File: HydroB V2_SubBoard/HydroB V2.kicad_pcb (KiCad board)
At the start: 4 copper layers, 89.6 x 101.8 mm, 77 parts, among them J1 FAN, J14 Screw_Terminal_01x02, J15 Screw_Terminal_01x02, J16 Screw_Terminal_01x02, J17 Screw_Terminal_01x02, J18 Screw_Terminal_01x02, J3 Conn_01x02_Pin, J4 Conn_01x04_Pin, J5 PH SENSOR, J6 EC SENSOR, J7 Conn_01x02_Pin, K10 SRD-05VDC-SL-C, K5 SRD-05VDC-SL-C, K7 SRD-05VDC-SL-C, K8 SRD-05VDC-SL-C, K9 SRD-05VDC-SL-C, Q10 S8050, Q6 S8050, Q7 S8050, Q8 S8050, Q9 S8050, SW1 SW_Push, U1 STM32F103C8Tx, U2 TPS5410D, U3 SN65HVD72DR, U4 TPS7A2633DRVR, U5 SN65HVD230, Y1 8Mhz

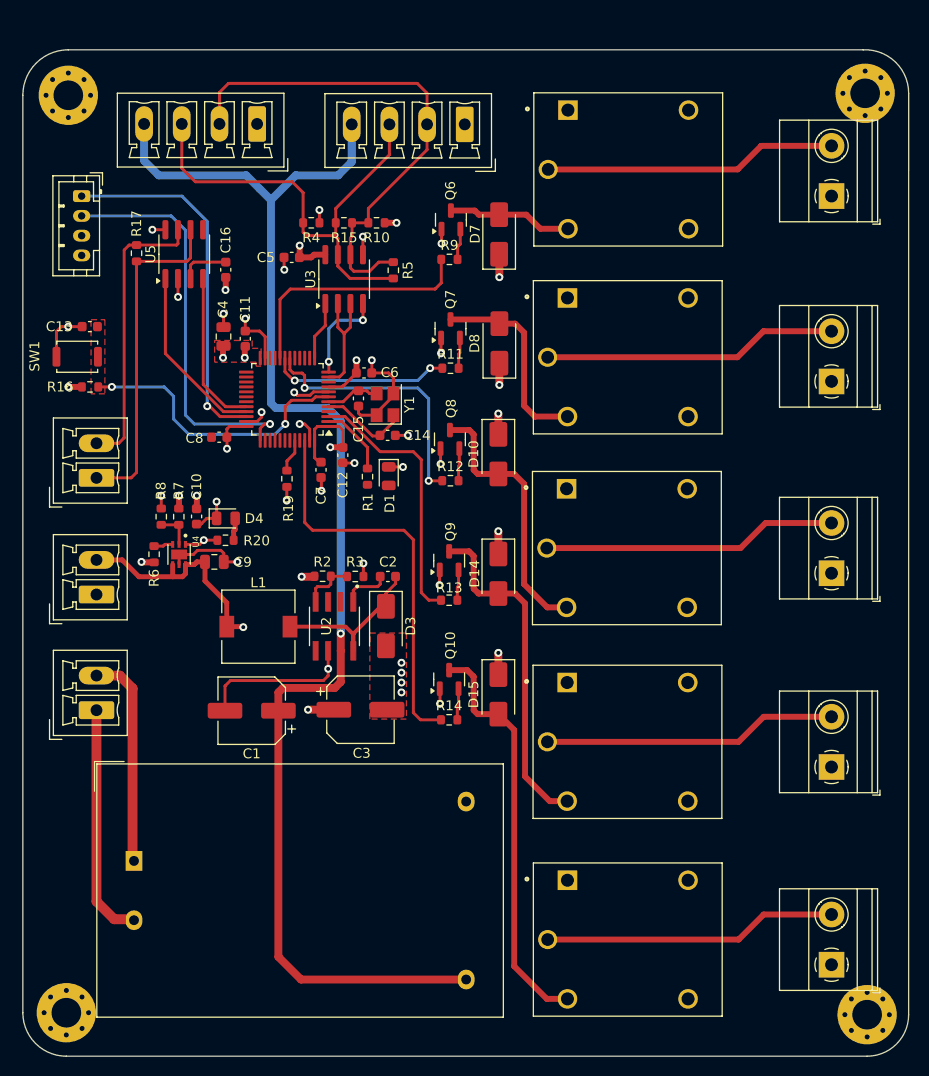
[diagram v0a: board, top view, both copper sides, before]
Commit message: finish the subboard layout
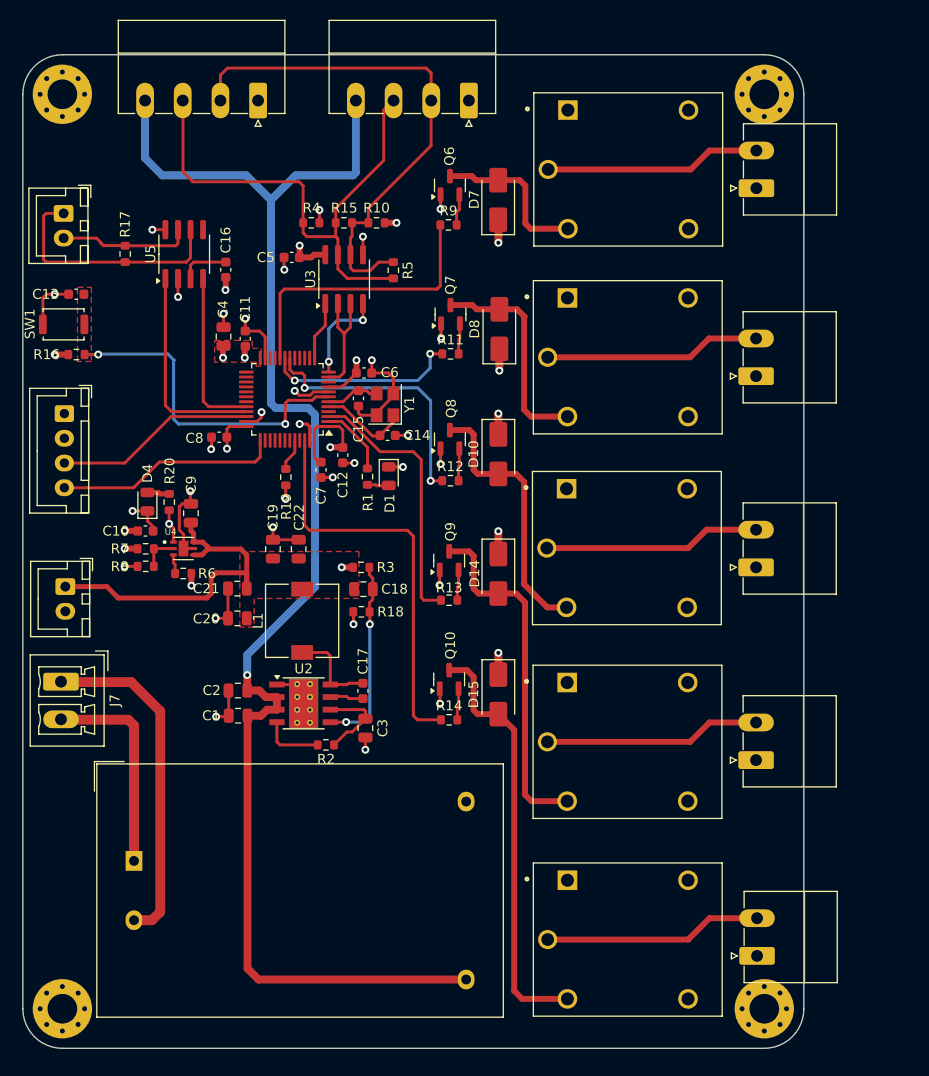
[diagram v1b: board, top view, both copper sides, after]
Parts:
- removed D3: B340, Diode_SMD:D_SMA
- removed J3: Conn_01x02_Pin, Connector_Phoenix_MC:PhoenixContact_MCV_1,5_2-G-3.5_1x02_P3.50mm_Vertical
- added C17: 0.1uF, Capacitor_SMD:C_0603_1608Metric, F.Cu at (138.4, 109.8)
- added C18: c, Capacitor_SMD:C_0805_2012Metric, F.Cu at (138.4, 99.6)
- added C19: 22uF, Capacitor_SMD:C_0805_2012Metric, F.Cu at (129.3, 95.5)
- added C20: 22uF, Capacitor_SMD:C_0805_2012Metric, F.Cu at (125.7, 102.5)
- added C21: 22uF, Capacitor_SMD:C_0805_2012Metric, F.Cu at (125.7, 99.5)
- added C22: 22uF, Capacitor_SMD:C_0805_2012Metric, F.Cu at (131.9, 95.5)
- added J2: Conn_01x02_Pin, Connector_JST:JST_XH_B2B-XH-A_1x02_P2.50mm_Vertical, F.Cu at (108.3, 99.3)
- added R18: 9.09k, Resistor_SMD:R_0603_1608Metric, F.Cu at (138.2, 101.8)
- C1: value 4.7uF -> 10uF; footprint Capacitor_SMD:CP_Elec_6.3x5.4_Nichicon -> Capacitor_SMD:C_0805_2012Metric
- C2: value 0.01uF -> 220nF; footprint Capacitor_SMD:C_0603_1608Metric -> Capacitor_SMD:C_0805_2012Metric
- C3: value 47uF -> 1uF; footprint Capacitor_SMD:CP_Elec_6.3x5.4_Nichicon -> Capacitor_SMD:C_0805_2012Metric
- J1: value FAN -> Conn_01x02_Pin; footprint Connector_Phoenix_MC:PhoenixContact_MCV_1,5_2-G-3.5_1x02_P3.50mm_Vertical -> Connector_JST:JST_XH_B2B-XH-A_1x02_P2.50mm_Vertical
- J14, J15, J16, J17, J18: footprint TerminalBlock_Phoenix:TerminalBlock_Phoenix_MKDS-1,5-2-5.08_1x02_P5.08mm_Horizontal -> Connector_Phoenix_MC:PhoenixContact_MC_1,5_2-G-3.81_1x02_P3.81mm_Horizontal
- J4: footprint Connector_JST:JST_PH_B4B-PH-K_1x04_P2.00mm_Vertical -> Connector_JST:JST_XH_B4B-XH-A_1x04_P2.50mm_Vertical
- J5, J6: footprint Connector_Phoenix_MC:PhoenixContact_MCV_1,5_4-G-3.81_1x04_P3.81mm_Vertical -> Connector_Phoenix_MC:PhoenixContact_MC_1,5_4-G-3.81_1x04_P3.81mm_Horizontal
- J7: footprint Connector_Phoenix_MC:PhoenixContact_MCV_1,5_2-G-3.5_1x02_P3.50mm_Vertical -> Connector_Phoenix_MC:PhoenixContact_MCV_1,5_2-G-3.81_1x02_P3.81mm_Vertical
- L1: value 68uH -> 27uH; footprint Inductor_SMD:L_7.3x7.3_H4.5 -> Inductor_SMD:L_7.3x7.3_H3.5
- R2: value 10k -> 100k
- R3: value 1.13k -> 100k
- U2: value TPS5410D -> LMR33620ADDA; footprint TPS5410D:SOIC127P599X175-8N -> Package_SO:Texas_HSOP-8-1EP_3.9x4.9mm_P1.27mm_ThermalVias
- moved J1 38.7 mm to (108.1, 61.5), turned to -90 degrees
- moved J4 22.1 mm to (108.2, 81.8)
- moved C2 19.1 mm to (125.8, 109.8)
- moved R2 17.1 mm to (134.7, 115.3), turned to 0 degrees
- moved H6 10.4 mm to (179.0, 142.0)
- moved H5 10.2 mm to (179.0, 49.5)
- moved U2 8.39 mm to (132.4, 111.1), turned to 0 degrees
- moved D4 8.11 mm to (116.6, 90.7), turned to 90 degrees
- moved J17 7.66 mm to (178.2, 116.8)
- moved J16 7.66 mm to (178.2, 97.3)
- moved J15 7.65 mm to (178.2, 78.0)
- moved J14 7.65 mm to (178.2, 59.0)
- moved J18 7.59 mm to (178.3, 136.7)
- moved R20 6.88 mm to (118.8, 90.8), turned to 90 degrees
- moved C9 5.47 mm to (121.0, 91.9), turned to 90 degrees
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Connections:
- C2 pad 1: Net-(D3-K) -> +24V
- C2 pad 2: Net-(U2-BOOT) -> GND
- C3 pad 1: +12V -> Net-(U2-VCC)
- J1 pad 1: GND -> Net-(J1-Pin_1)
- J1 pad 2: +12V -> Net-(J1-Pin_2)
- J4 pad 1: SWDIO -> GND
- J4 pad 2: SWCLK -> +3.3V
- J4 pad 3: +3.3V -> SWDIO
- J4 pad 4: GND -> SWCLK
- L1 pad 1: +12V -> Net-(U2-SW)
- L1 pad 2: Net-(D3-K) -> +12V
- R17 pad 1: Net-(J3-Pin_1) -> Net-(J1-Pin_1)
- R17 pad 2: Net-(J3-Pin_2) -> Net-(J1-Pin_2)
- R2 pad 1: Net-(U2-VSENSE) -> PG
- R2 pad 2: +12V -> Net-(U2-VCC)
- R3 pad 1: GND -> Net-(U2-FB)
- R3 pad 2: Net-(U2-VSENSE) -> +12V
- U2 pad 1: Net-(U2-BOOT) -> GND
- U2 pad 2: (no net) -> +24V
- U2 pad 3: (no net) -> +24V
- U2 pad 4: Net-(U2-VSENSE) -> PG
- U2 pad 5: ENA -> Net-(U2-FB)
- U2 pad 6: GND -> Net-(U2-VCC)
- U2 pad 7: +24V -> Net-(U2-BOOT)
- U2 pad 8: Net-(D3-K) -> Net-(U2-SW)
- U5 pad 6: Net-(J3-Pin_1) -> Net-(J1-Pin_1)
- U5 pad 7: Net-(J3-Pin_2) -> Net-(J1-Pin_2)
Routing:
- net Net-(J3-Pin_1): track 34.1 -> 0.00 mm
- net Net-(J3-Pin_2): track 29.1 -> 0.00 mm
- net Net-(J1-Pin_1): track 0.00 -> 24.5 mm
- net Net-(U2-FB): track 0.00 -> 19.8 mm, vias 0 -> 2
- net Net-(D3-K): track 18.4 -> 0.00 mm
- net SWCLK: track 41.1 -> 23.5 mm, vias 1 -> 0
- net SWDIO: track 36.8 -> 20.3 mm, vias 1 -> 0
- net Net-(J1-Pin_2): track 0.00 -> 13.4 mm
- net N: track 23.3 -> 34.6 mm
- net +24V: track 139.8 -> 149.6 mm
- net +12V: track 38.3 -> 48.0 mm, vias 8 -> 6
- net Net-(U2-SW): track 0.00 -> 9.25 mm
- net Net-(U2-VCC): track 0.00 -> 8.65 mm
- net Net-(J17-Pin_2): track 29.8 -> 21.8 mm
- net Net-(J15-Pin_2): track 29.8 -> 22.1 mm
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- added copper zone on F.Cu, net +12V
- removed copper zone on F.Cu, net GND
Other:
- board size 89.6 x 101.8 mm -> 79 x 100.5 mm
